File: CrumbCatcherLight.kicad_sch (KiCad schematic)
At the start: 1 part, among them U0 PCB

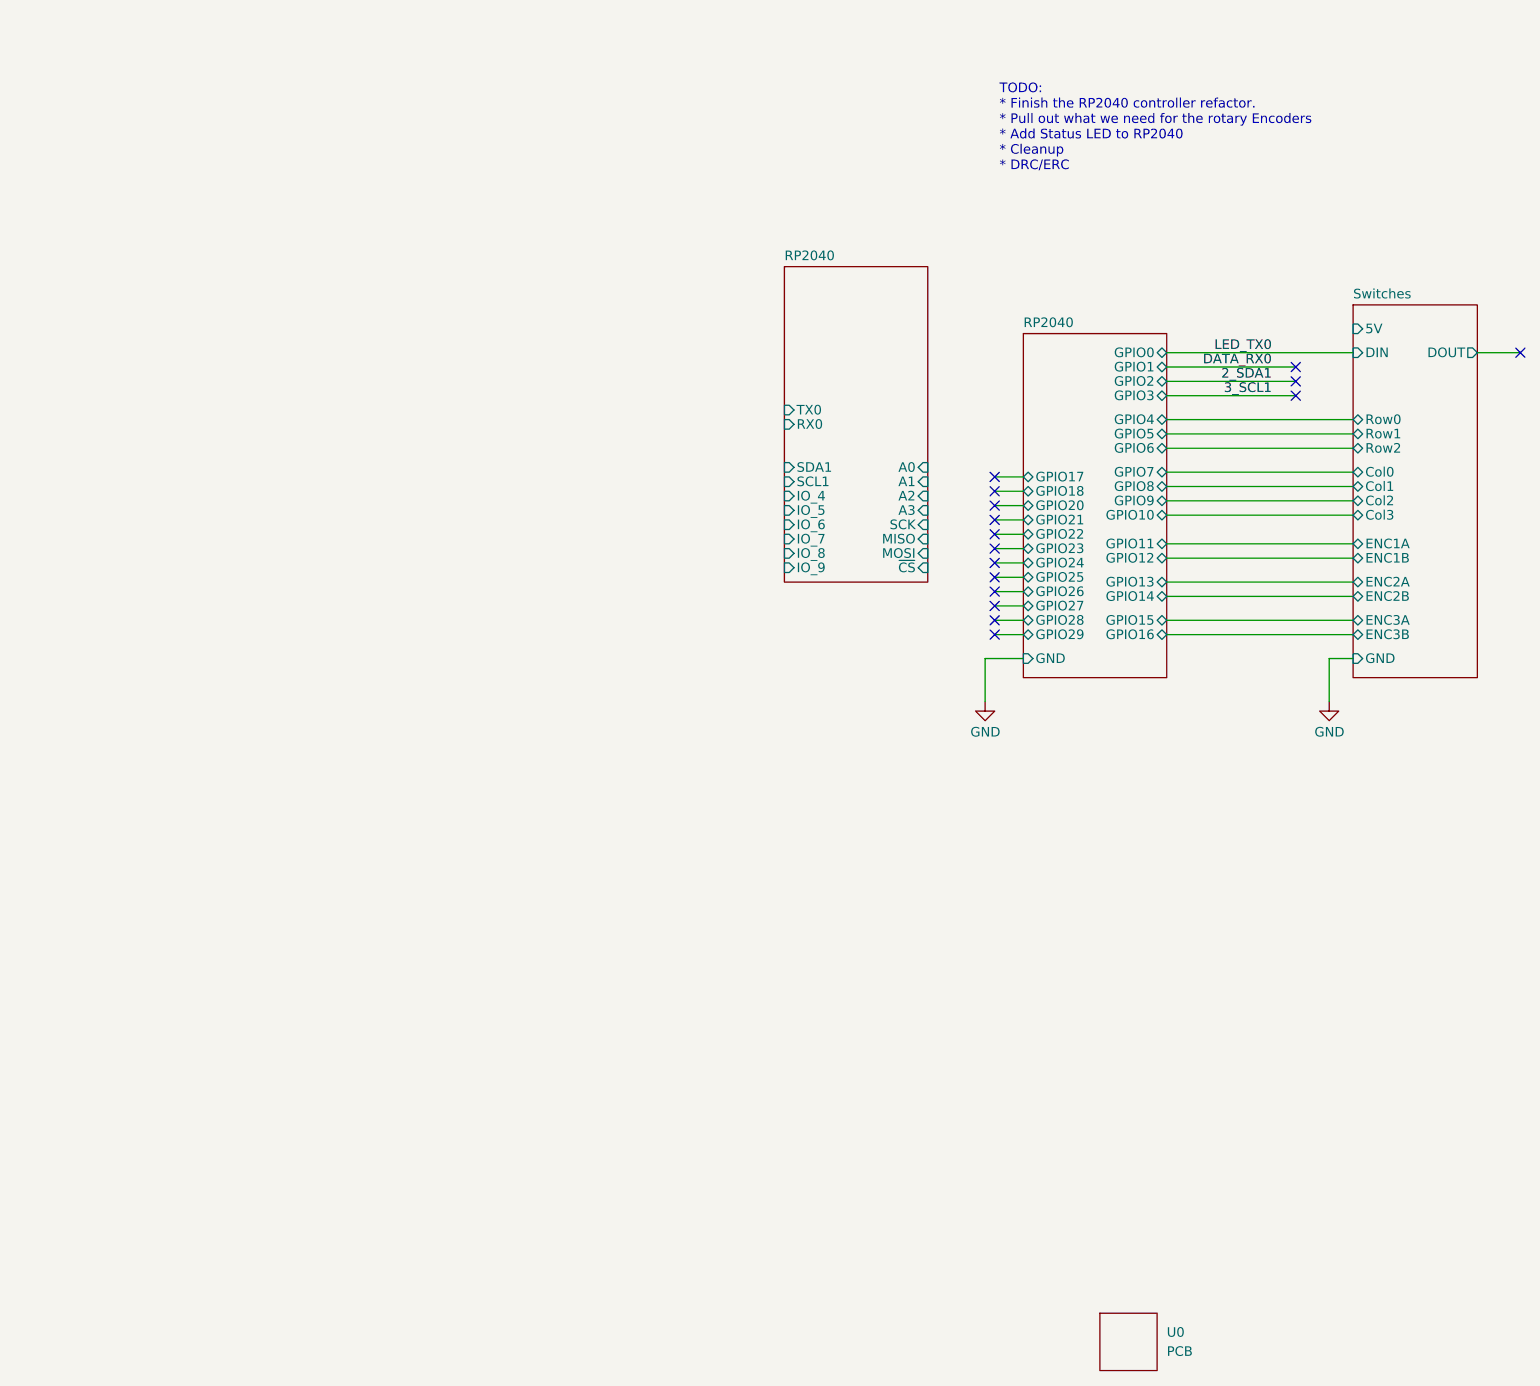
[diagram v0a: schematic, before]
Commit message: Update BOM,
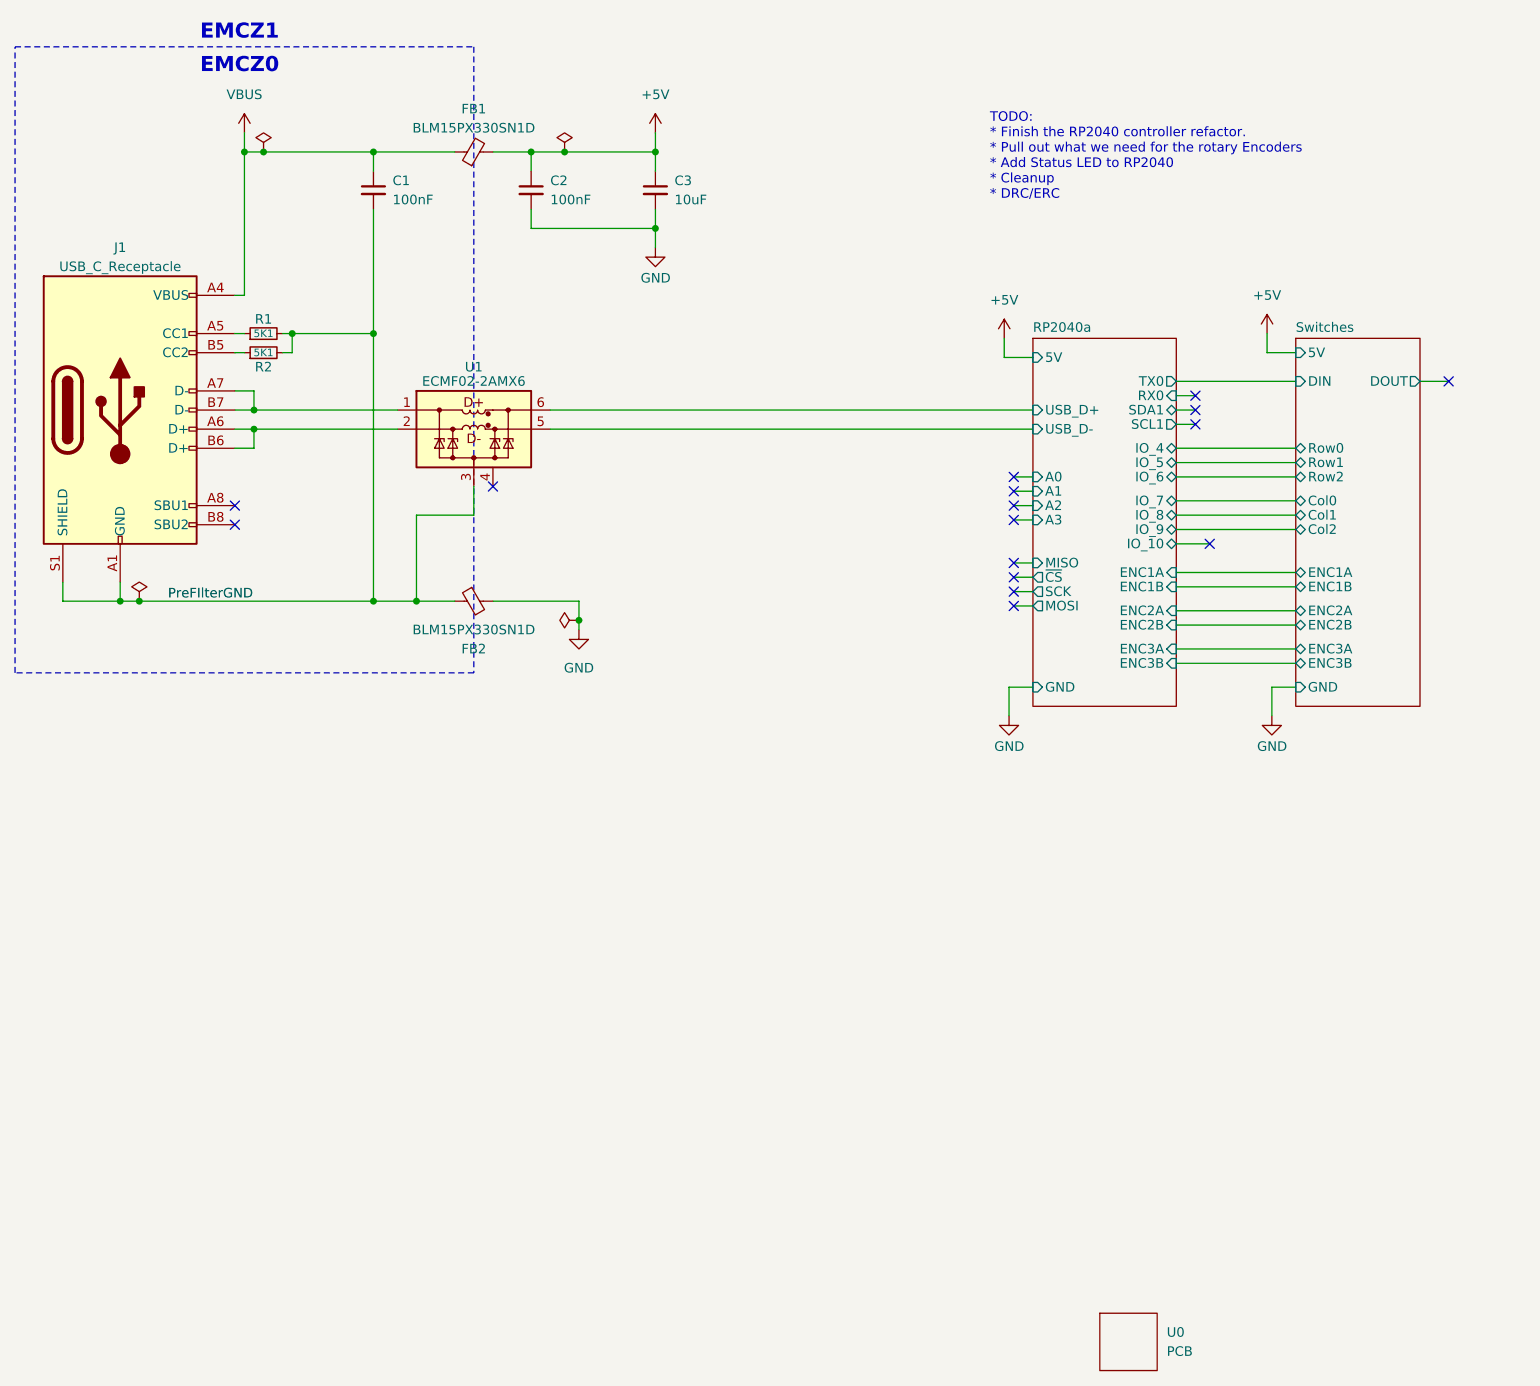
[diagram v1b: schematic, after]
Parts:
- added C1, C2: 100nF, Capacitor_SMD:C_0402_1005Metric, symbol Device:C_Small
- added C3: 10uF, Capacitor_SMD:C_0805_2012Metric, symbol Device:C_Small
- added FB1, FB2: BLM15PX330SN1D, Inductor_SMD:L_0402_1005Metric, symbol Device:FerriteBead_Small
- added J1: USB_C_Receptacle, Connector_USB:USB_C_Receptacle_GCT_USB4105-xx-A_16P_TopMnt_Horizontal, symbol Connector:USB_C_Receptacle_USB2.0_16P
- added R1, R2: 5K1, Resistor_SMD:R_0402_1005Metric, symbol Device:R_Small
- added U1: ECMF02-2AMX6, Package_DFN_QFN:ST_UQFN-6L_1.5x1.7mm_P0.5mm, symbol Power_Protection:ECMF02-2AMX6
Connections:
- net GND: now also C2.2, C3.2, FB2.2
- new net: J1.A5 (CC1), R1.1
- new net: J1.A6 (D+), J1.B6 (D+), U1.2 (D-_in)
- new net: J1.A7 (D-), J1.B7 (D-), U1.1 (D+_in)
- new net: J1.B5 (CC2), R2.1
- new net +5V: C2.1, C3.1, FB1.2
- new net PreFIlterGND: C1.2, FB2.1, J1.A1 (GND), J1.A12 (GND), J1.B1 (GND), J1.B12 (GND), J1.S1 (SHIELD), R1.2, R2.2, U1.3 (GND)
- new net RP2040a/USB_D+: U1.6 (D+_out)
- new net RP2040a/USB_D-: U1.5 (D-_out)
- new net VBUS: C1.1, FB1.1, J1.A4 (VBUS), J1.A9 (VBUS), J1.B4 (VBUS), J1.B9 (VBUS)
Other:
- removed sheet RP2040
- added sheet RP2040a (mad_lib/schematics/Keyboard Controllers/RP2040.kicad_sch)
- sheet Switches ports: added none; removed Col3
- note added: "EMCZ0"
- note added: "EMCZ1"
